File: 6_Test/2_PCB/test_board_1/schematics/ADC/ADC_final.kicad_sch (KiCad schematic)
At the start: 2 parts

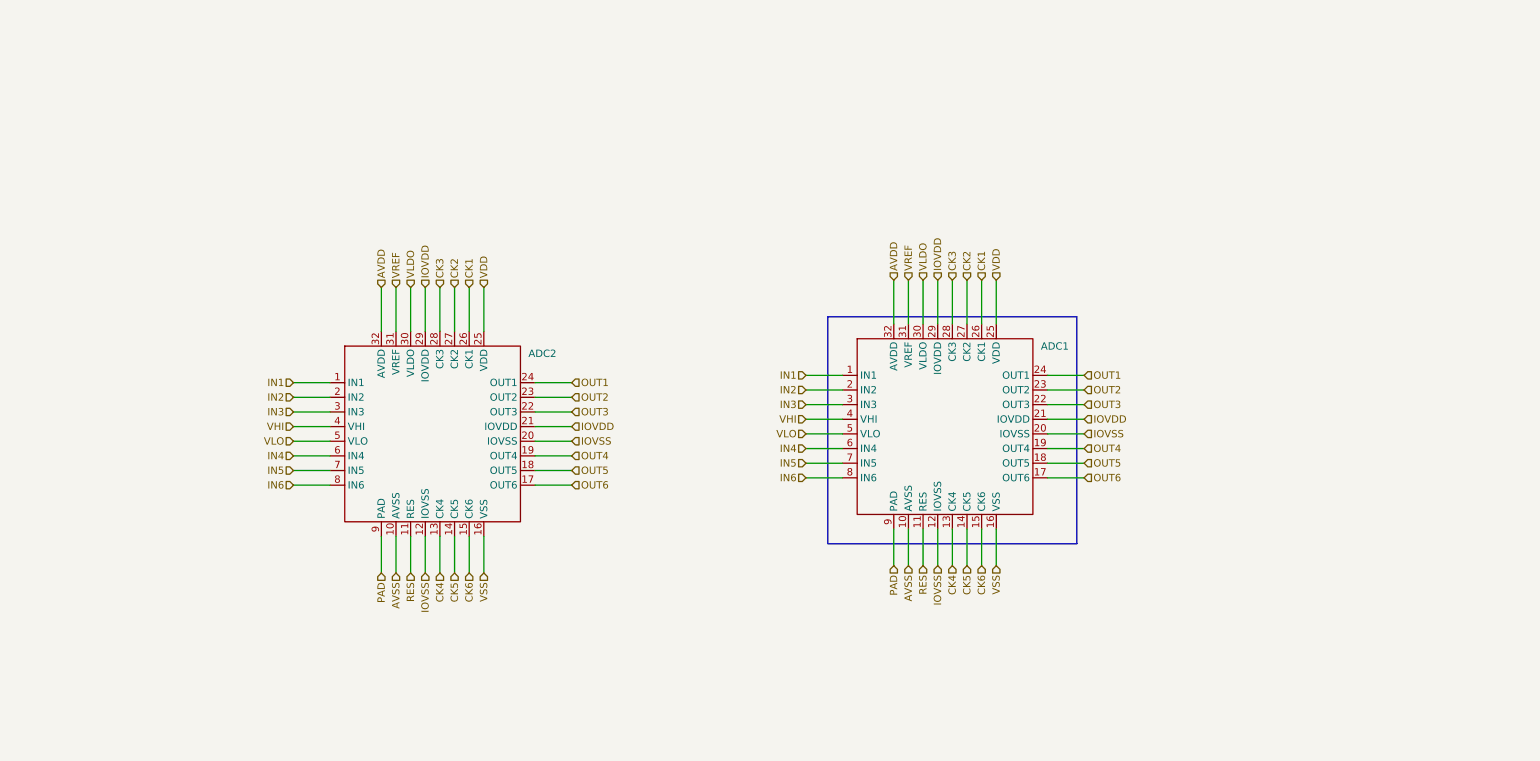
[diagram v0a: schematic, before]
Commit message: final draft of board done.
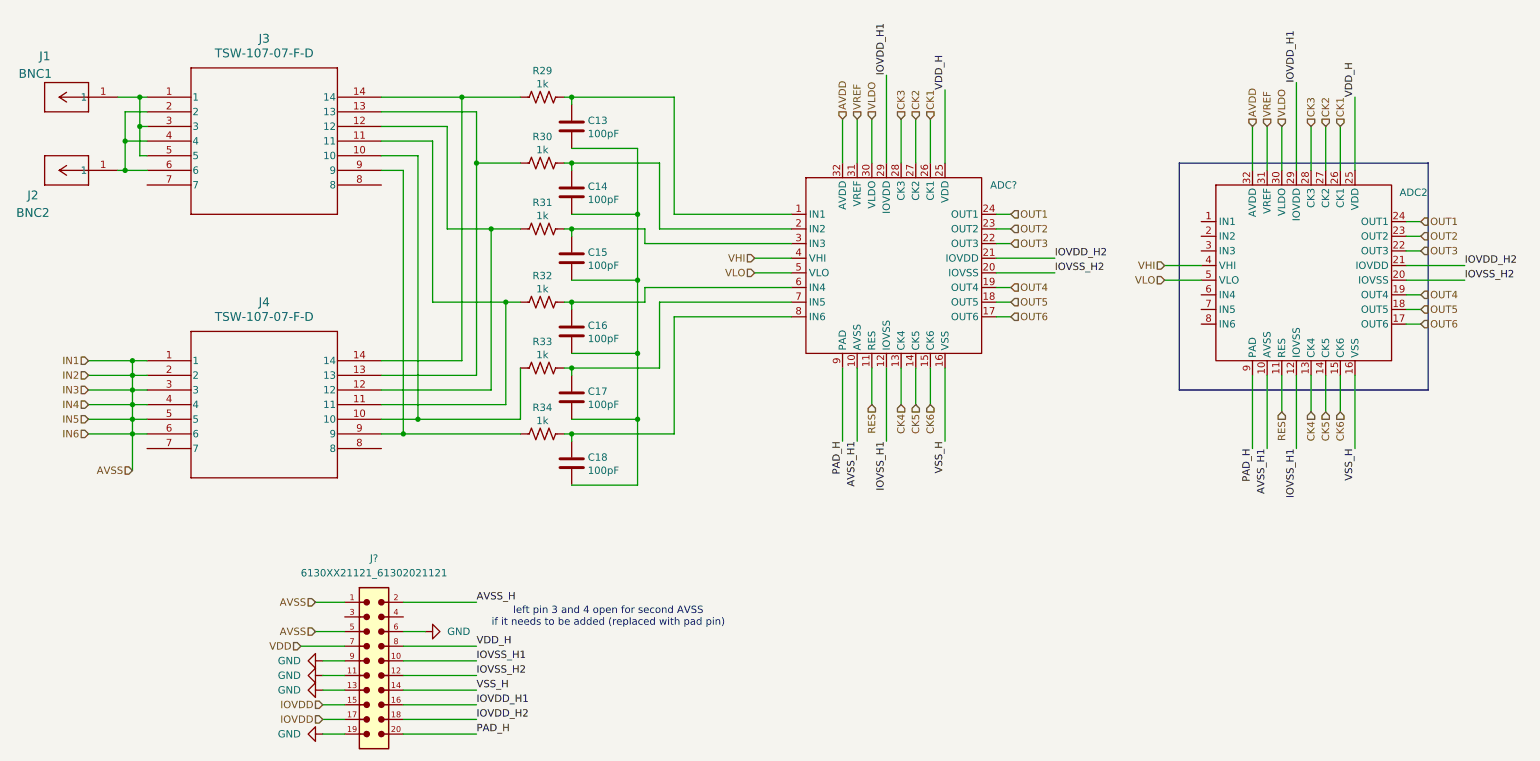
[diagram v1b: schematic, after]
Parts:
- removed ADC1: ~, Package_DIP:DIP-32_W15.24mm_Socket, symbol ADC:Chip
- added ADC2: ~, Package_DFN_QFN:QFN-32-1EP_5x5mm_P0.5mm_EP3.1x3.1mm_ThermalVias, symbol ADC:Chip
- added C13, C14, C15, C16, C17, C18: 100pF, symbol Device:C
- added J1: BNC1, CONN_1274571-1_TYCO, symbol bnc_mini:1274571-1
- added J2: BNC2, CONN_1274571-1_TYCO, symbol bnc_mini:1274571-1
- added J3, J4: TSW-107-07-F-D, TSW-107-07-G-D_SAI, symbol 6x2Header:TSW-107-07-F-D
- added J?: 6130XX21121_61302021121, 6130XX21121_61302021121:61302021121, symbol 2x10Header:6130XX21121_61302021121
- added R29, R30, R31, R32, R33, R34: 1k, symbol Device:R_US
- ADC?: renamed from ADC2; footprint Package_DIP:DIP-32_W15.24mm_Socket -> Package_DFN_QFN:QFN-32-1EP_5x5mm_P0.5mm_EP3.1x3.1mm_ThermalVias; now left out of the parts list
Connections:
- net AVDD: now also ADC2.32 (AVDD)
- net AVSS: now also J4.1, J4.2, J4.3, J4.4, J4.5, J4.6, J?.1, J?.5; no longer ADC?.10 (AVSS)
- net CK1: now also ADC2.26 (CK1)
- net CK2: now also ADC2.27 (CK2)
- net CK3: now also ADC2.28 (CK3)
- net CK4: now also ADC2.13 (CK4)
- net CK5: now also ADC2.14 (CK5)
- net CK6: now also ADC2.15 (CK6)
- net IOVDD: now also J?.15, J?.17; no longer ADC?.21 (IOVDD), ADC?.29 (IOVDD)
- net OUT1: now also ADC2.24 (OUT1)
- net OUT2: now also ADC2.23 (OUT2)
- net OUT3: now also ADC2.22 (OUT3)
- net OUT4: now also ADC2.19 (OUT4)
- net OUT5: now also ADC2.18 (OUT5)
- net OUT6: now also ADC2.17 (OUT6)
- net RES: now also ADC2.11 (RES)
- net VDD: now also J?.7; no longer ADC?.25 (VDD)
- net VHI: now also ADC2.4 (VHI)
- net VLDO: now also ADC2.30 (VLDO)
- net VLO: now also ADC2.5 (VLO)
- net VREF: now also ADC2.31 (VREF)
- net IN1: no longer names the net of ADC?.1 (IN1)
- net IN1: now also C13.1, R29.2
- net IN2: no longer names the net of ADC?.2 (IN2)
- net IN2: now also C14.1, R30.2
- net IN3: no longer names the net of ADC?.3 (IN3)
- net IN3: now also C15.1, R31.2
- net IN4: no longer names the net of ADC?.6 (IN4)
- net IN4: now also C16.1, R32.2
- net IN5: no longer names the net of ADC?.7 (IN5)
- net IN5: now also C17.1, R33.2
- net IN6: no longer names the net of ADC?.8 (IN6)
- net IN6: now also C18.1, R34.2
- net IOVSS renamed IOVSS_H1
- net IOVSS_H1: now also ADC2.12 (IOVSS), J?.10; no longer ADC?.20 (IOVSS)
- net PAD renamed PAD_H
- net PAD_H: now also ADC2.9 (PAD), J?.20
- net VSS renamed VSS_H
- net VSS_H: now also ADC2.16 (VSS), J?.14
- new net: J3.10, J4.10, R33.1
- new net: J3.13, J4.13, R30.1
- new net: J3.11, J4.11, R32.1
- new net: C13.2, C14.2, C15.2, C16.2, C17.2, C18.2
- new net: J1.1, J3.1, J3.3, J3.5
- new net: J3.12, J4.12, R31.1
- new net: J3.14, J4.14, R29.1
- new net: J2.1, J3.2, J3.4, J3.6
- new net: J3.9, J4.9, R34.1
- new net AVSS_H: J?.2
- new net AVSS_H1: ADC2.10 (AVSS), ADC?.10 (AVSS)
- new net GND: J?.11, J?.13, J?.19, J?.6, J?.9
- new net IOVDD_H1: ADC2.29 (IOVDD), ADC?.29 (IOVDD), J?.16
- new net IOVDD_H2: ADC2.21 (IOVDD), ADC?.21 (IOVDD), J?.18
- new net IOVSS_H2: ADC2.20 (IOVSS), ADC?.20 (IOVSS), J?.12
- new net VDD_H: ADC2.25 (VDD), ADC?.25 (VDD), J?.8
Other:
- note added: "left pin 3 and 4 open for second AVSS if it needs to be added (replaced with pad pin)"
- moved on the sheet: ADC?
